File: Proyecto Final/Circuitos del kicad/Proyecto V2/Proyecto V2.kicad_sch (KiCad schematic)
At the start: 40 parts, among them J1 12v, J2 I2C + LCD, J3 DS1307, J4 Encoder, J5 Conn_01x02, J6 Conn_01x02, J7 Conn_01x02, J8 Conn_01x05, J9 Conn_01x05, K1 RAYEX-L90, K2 RAYEX-L90, K3 RAYEX-L90, Q1 PN2222A, Q2 PN2222A, Q3 PN2222A, SW1 SW_Push, SW2 SW_Push, SW3 SW_Push, SW4 SW_Push, U1 LM7805, U3 ATmega328P-P, U4 NodeMCU1.0(ESP-12E), Y1 16MHz

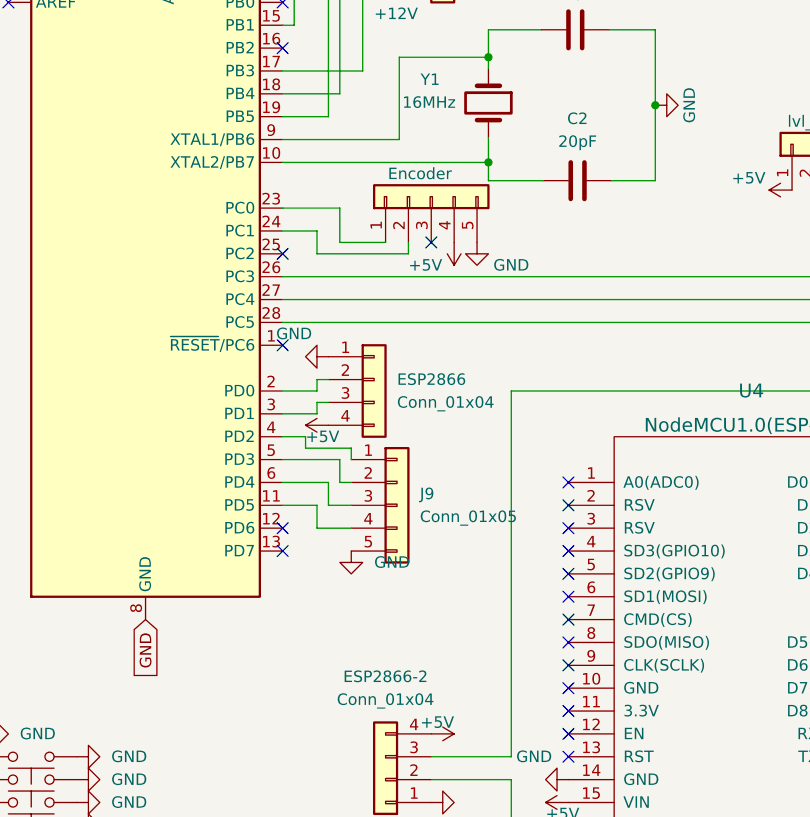
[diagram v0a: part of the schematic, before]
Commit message: SEXOOO
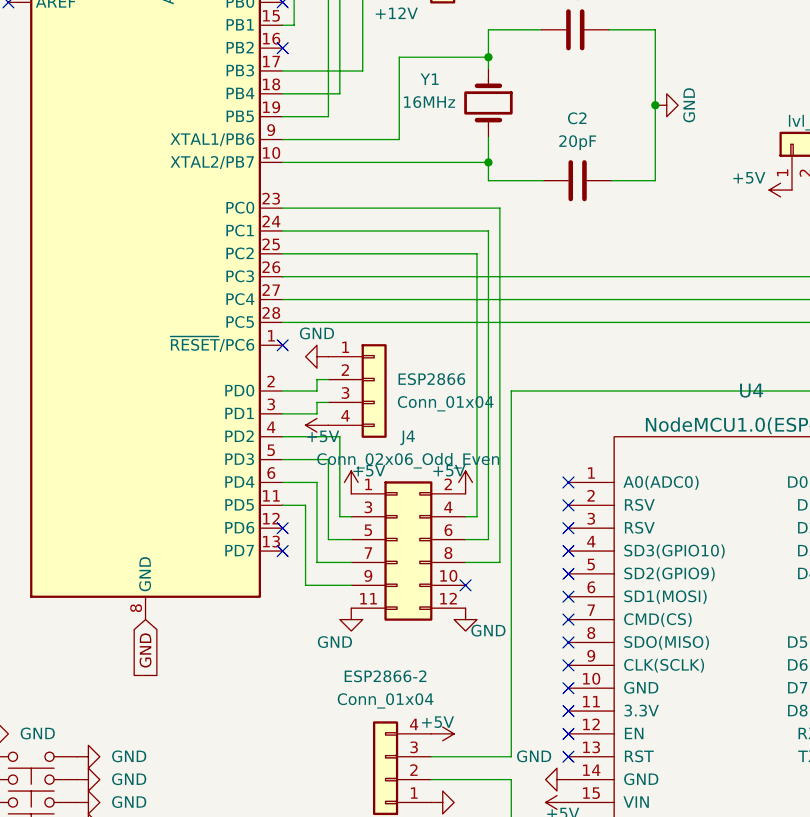
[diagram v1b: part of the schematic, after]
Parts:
- removed J4: Encoder, Connector_PinSocket_2.54mm:PinSocket_1x05_P2.54mm_Vertical, symbol Connector_Generic:Conn_01x05
- removed J9: Conn_01x05, Connector_PinHeader_2.54mm:PinHeader_1x05_P2.54mm_Vertical, symbol Connector_Generic:Conn_01x05
- added J4: Conn_02x06_Odd_Even, Connector_PinHeader_2.54mm:PinHeader_2x06_P2.54mm_Vertical, symbol Connector_Generic:Conn_02x06_Odd_Even
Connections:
- net +5V: now also J4.1 (Pin_1), J4.2 (Pin_2)
- net GND: now also J4.11 (Pin_11), J4.12 (Pin_12)
- net at U3.23 (PC0): now also J4.8 (Pin_8)
- net at U3.24 (PC1): now also J4.6 (Pin_6)
- net at U3.4 (PD2): now also J4.3 (Pin_3)
- net at U3.5 (PD3): now also J4.5 (Pin_5)
- net at U3.6 (PD4): now also J4.7 (Pin_7)
- net at U3.11 (PD5): now also J4.9 (Pin_9)
- net at U3.25 (PC2): now also J4.4 (Pin_4)
- no-connect marks 34 -> 33
